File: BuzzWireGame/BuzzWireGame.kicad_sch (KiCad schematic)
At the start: 10 parts, among them J1 Wire track terminal, U1 NE555P

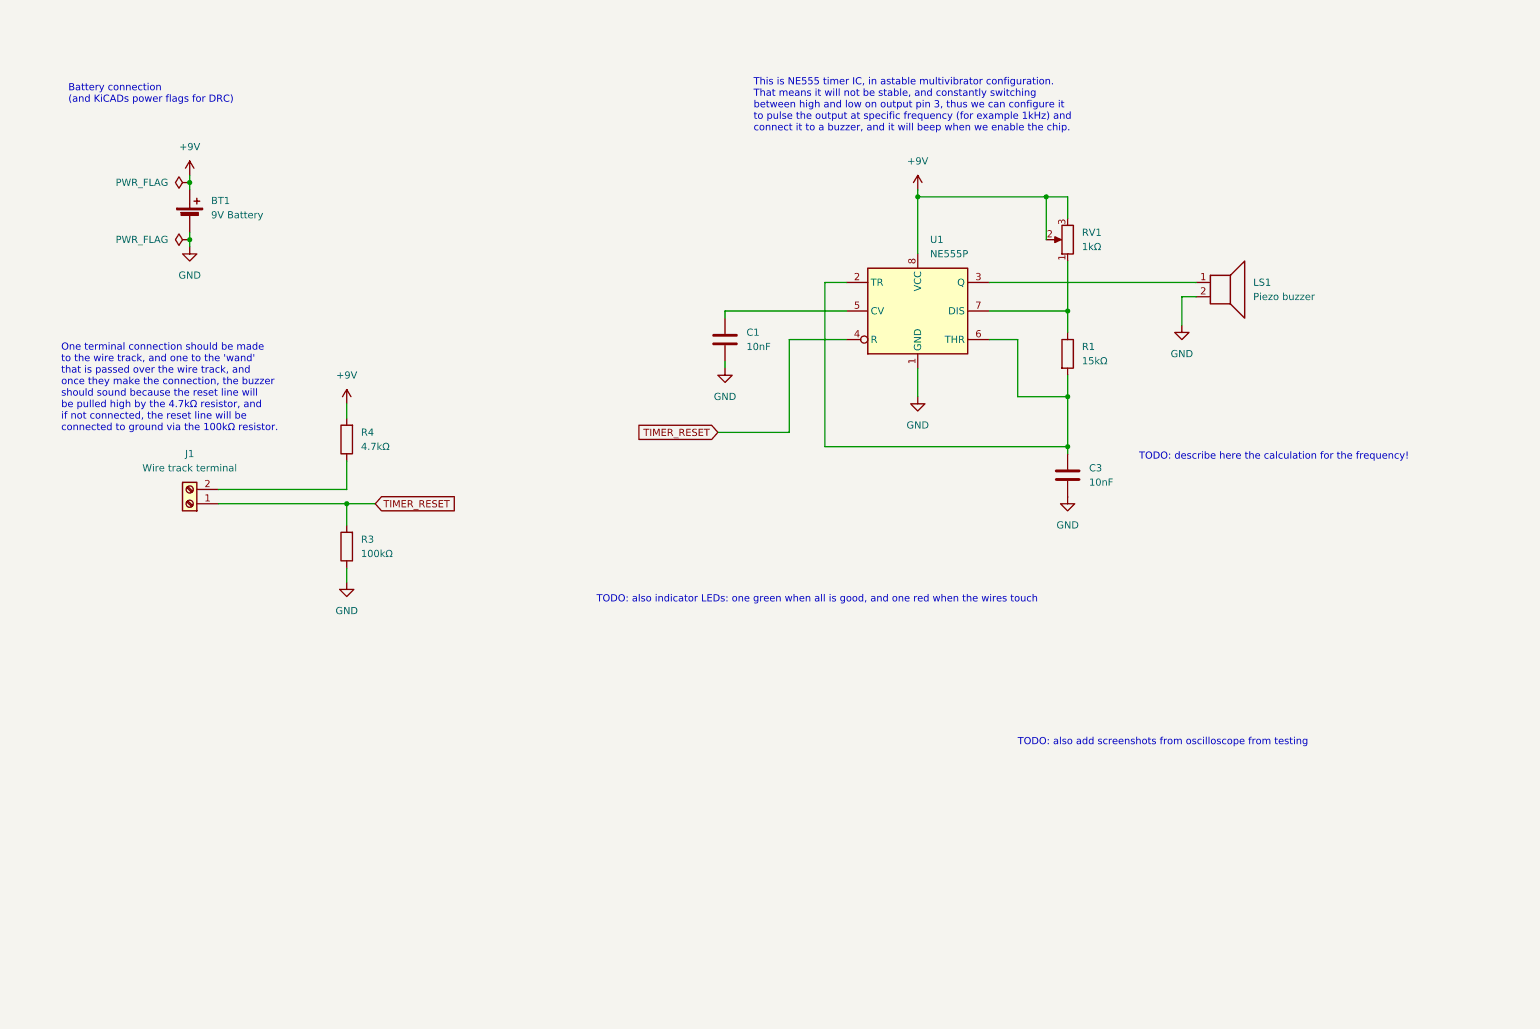
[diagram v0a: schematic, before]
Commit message: Finish schm and PCB design for v1.0
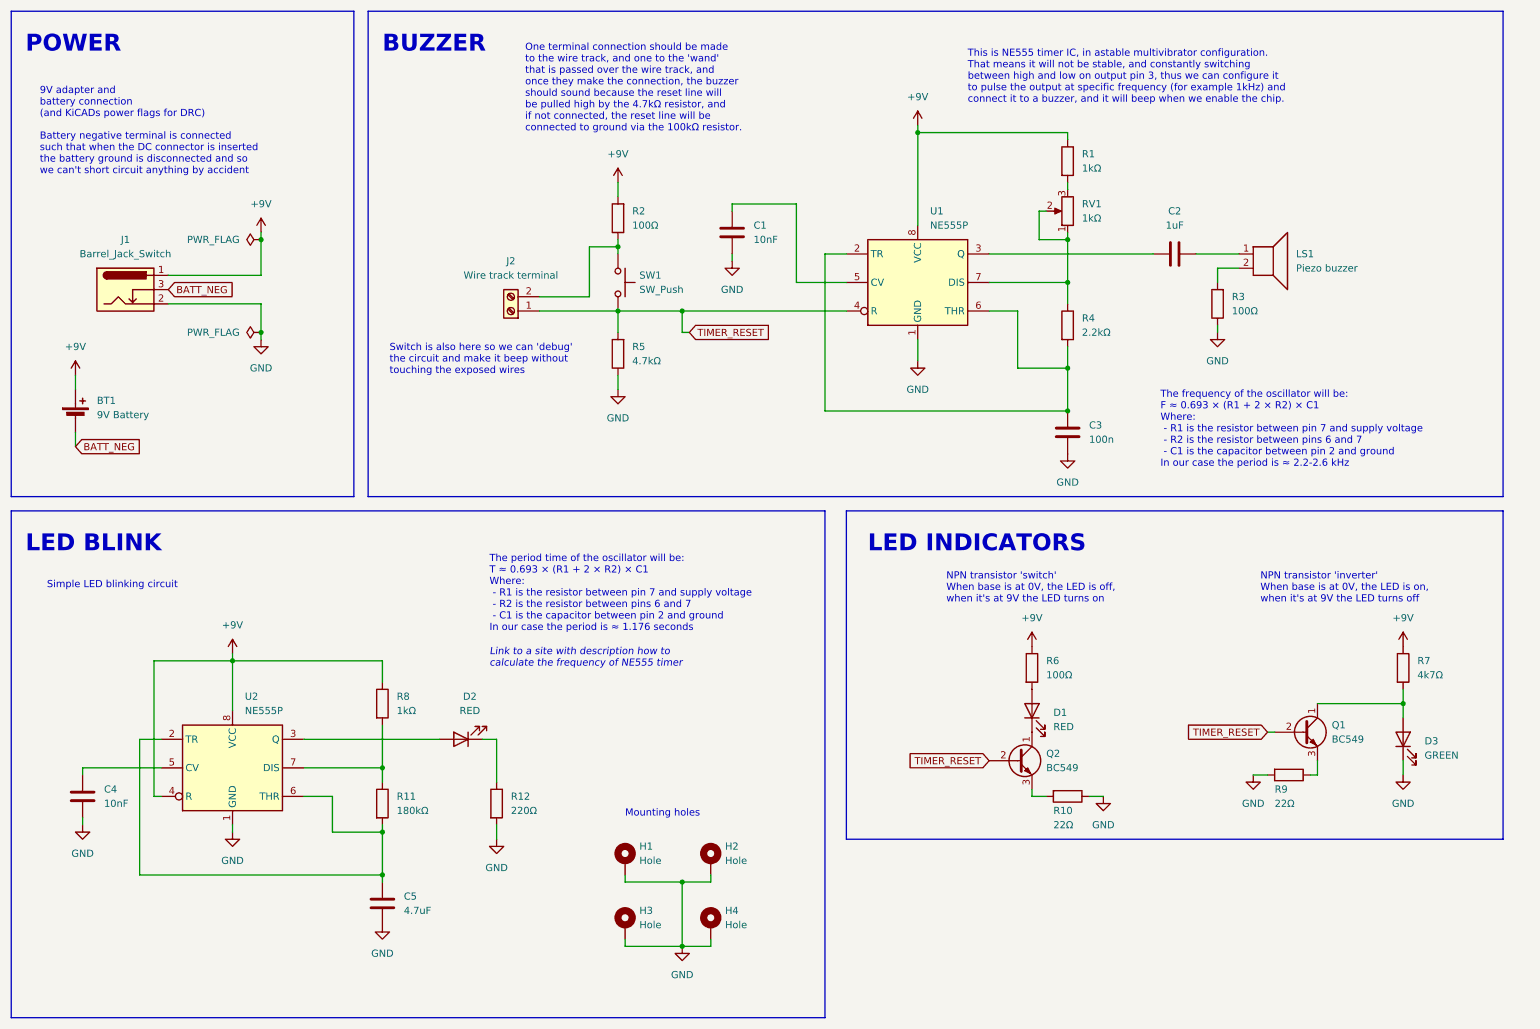
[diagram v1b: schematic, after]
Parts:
- removed R4: 4.7kΩ, Resistor_THT:R_Axial_DIN0207_L6.3mm_D2.5mm_P7.62mm_Horizontal, symbol Device:R
- added C2: 1uF, Capacitor_SMD:C_1206_3216Metric, symbol Device:C
- added C4: 10nF, Capacitor_SMD:C_1206_3216Metric, symbol Device:C
- added C5: 4.7uF, Capacitor_THT:CP_Radial_D4.0mm_P2.00mm, symbol Device:C
- added D1, D2: RED, LED_THT:LED_D5.0mm_Clear, symbol Device:LED
- added D3: GREEN, LED_THT:LED_D5.0mm_Clear, symbol Device:LED
- added H1, H2, H3, H4: Hole, MountingHole:MountingHole_3.2mm_M3_Pad_Via, symbol Mechanical:MountingHole_Pad
- added J1: Barrel_Jack_Switch, Connector_BarrelJack:BarrelJack_Horizontal, symbol Connector:Barrel_Jack_Switch
- added Q1, Q2: BC549, Package_TO_SOT_THT:TO-92_Inline, symbol Transistor_BJT:BC549
- added R1, R8: 1kΩ, Resistor_THT:R_Axial_DIN0207_L6.3mm_D2.5mm_P10.16mm_Horizontal, symbol Device:R
- added R10, R9: 22Ω, Resistor_THT:R_Axial_DIN0207_L6.3mm_D2.5mm_P10.16mm_Horizontal, symbol Device:R
- added R11: 180kΩ, Resistor_THT:R_Axial_DIN0207_L6.3mm_D2.5mm_P10.16mm_Horizontal, symbol Device:R
- added R12: 220Ω, Resistor_THT:R_Axial_DIN0207_L6.3mm_D2.5mm_P10.16mm_Horizontal, symbol Device:R
- added R2, R3, R6: 100Ω, Resistor_THT:R_Axial_DIN0207_L6.3mm_D2.5mm_P10.16mm_Horizontal, symbol Device:R
- added R7: 4k7Ω, Resistor_THT:R_Axial_DIN0207_L6.3mm_D2.5mm_P10.16mm_Horizontal, symbol Device:R
- added SW1: SW_Push, Button_Switch_THT:SW_PUSH_6mm_H4.3mm, symbol Switch:SW_Push
- added U2: NE555P, Package_DIP:DIP-8_W7.62mm, symbol Timer:NE555P
- BT1: footprint (none) -> TerminalBlock:TerminalBlock_bornier-2_P5.08mm
- C1: footprint (none) -> Capacitor_SMD:C_1206_3216Metric
- C3: value 10nF -> 100n; footprint (none) -> Capacitor_SMD:C_1206_3216Metric
- J2: renamed from J1; footprint (none) -> TerminalBlock:TerminalBlock_bornier-2_P5.08mm
- LS1: footprint (none) -> Buzzer_Beeper:Indicator_PUI_AI-1440-TWT-24V-2-R
- R4: renamed from R1; value 15kΩ -> 2.2kΩ; footprint Resistor_THT:R_Axial_DIN0207_L6.3mm_D2.5mm_P7.62mm_Horizontal -> Resistor_THT:R_Axial_DIN0207_L6.3mm_D2.5mm_P10.16mm_Horizontal
- R5: renamed from R3; value 100kΩ -> 4.7kΩ; footprint Resistor_THT:R_Axial_DIN0207_L6.3mm_D2.5mm_P7.62mm_Horizontal -> Resistor_THT:R_Axial_DIN0207_L6.3mm_D2.5mm_P10.16mm_Horizontal
- RV1: footprint (none) -> Potentiometer_THT:Potentiometer_Alps_RK163_Single_Horizontal
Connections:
- net +9V: now also J1.1, R1.1, R2.2, R6.1, R7.1, R8.1, U2.4 (R), U2.8 (VCC); no longer RV1.2, RV1.3
- net GND: now also C4.2, C5.2, D3.1 (K), H1.1, H2.1, H3.1, H4.1, J1.2, R10.1, R12.2, R3.1, R9.2, U2.1 (GND); no longer BT1.2 (-), LS1.2
- net TIMER_RESET: now also Q1.2 (B), Q2.2 (B), SW1.2
- net at R4.1, RV1.1, U1.7 (DIS): now also RV1.2
- net at J2.2 (Pin_2): now also R2.1, SW1.1
- net at U1.3 (Q): now also C2.1; no longer LS1.1
- new net: C2.2, LS1.1
- new net: R1.2, RV1.3
- new net: D1.1 (K), Q2.1 (C)
- new net: D1.2 (A), R6.2
- new net: Q2.3 (E), R10.2
- new net: Q1.3 (E), R9.1
- new net: C5.1, R11.2, U2.2 (TR), U2.6 (THR)
- new net: D2.2 (A), U2.3 (Q)
- new net: C4.1, U2.5 (CV)
- new net: R11.1, R8.2, U2.7 (DIS)
- new net: LS1.2, R3.2
- new net: D2.1 (K), R12.1
- new net: D3.2 (A), Q1.1 (C), R7.2
- new net BATT_NEG: BT1.2 (-), J1.3
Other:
- note added: "9V adapter and battery connection (and KiCADs power flags for DRC)"
- note added: "BUZZER"
- note added: "Battery negative terminal is connected such that when the DC connector is inserted the battery ground is disconnected and so we can't short circuit anything by accident"
- note added: "LED BLINK"
- note added: "LED INDICATORS"
- note added: "Link to a site with description how to calculate the frequency of NE555 timer"
- note added: "Mounting holes"
- note added: "NPN transistor 'inverter' When base is at 0V, the LED is on, when it's at 9V the LED turns off"
- note added: "NPN transistor 'switch' When base is at 0V, the LED is off, when it's at 9V the LED turns on"
- note added: "POWER"
- note added: "Simple LED blinking circuit"
- note added: "Switch is also here so we can 'debug' the circuit and make it beep without touching the exposed wires"
- note added: "The frequency of the oscillator will be: F ≈ 0.693 × (R1 + 2 × R2) × C1 Where: - R1 is the resistor between pin 7 and supply voltage - R2 is the resistor between pins 6 and 7 - C1 is the capacitor between pin 2 and ground In our case the period is ≈ 2.2-2.6 kHz"
- note added: "The period time of the oscillator will be: T ≈ 0.693 × (R1 + 2 × R2) × C1 Where: - R1 is the resistor between pin 7 and supply voltage - R2 is the resistor between pins 6 and 7 - C1 is the capacitor between pin 2 and ground In our case the period is ≈ 1.176 seconds"
- note removed: "Battery connection (and KiCADs power flags for DRC)"
- note removed: "TODO: also add screenshots from oscilloscope from testing"
- note removed: "TODO: also indicator LEDs: one green when all is good, and one red when the wires touch"
- note removed: "TODO: describe here the calculation for the frequency!"
- moved on the sheet: BT1, C1, C3, J2, LS1, R4, R5, RV1, U1
